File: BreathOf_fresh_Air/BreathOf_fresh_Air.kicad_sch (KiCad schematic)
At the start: 1 part, among them J1 4P4C

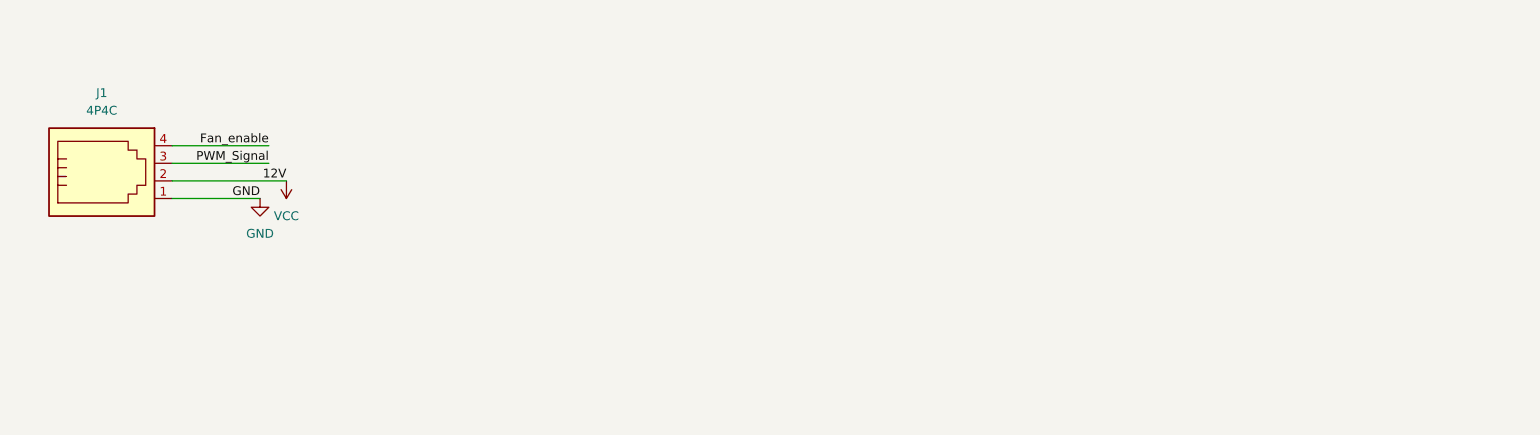
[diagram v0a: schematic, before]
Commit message: breath of fresh air
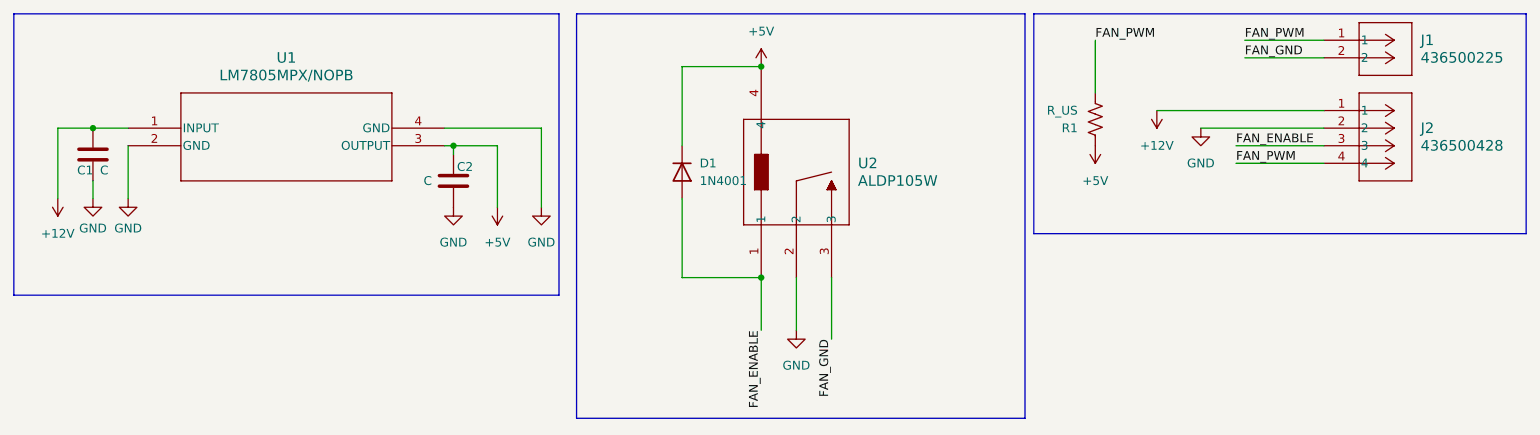
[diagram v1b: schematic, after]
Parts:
- removed J1: 4P4C, symbol Connector:4P4C
- added C1, C2: C, symbol Device:C
- added D1: 1N4001, Diode_THT:D_DO-41_SOD81_P10.16mm_Horizontal, symbol Diode:1N4001
- added J1: 436500225, CONN_SD-43650-009_02_MOL, symbol 43650-0225:436500225
- added J2: 436500428, CONN_SD-43650-010_04_MOL, symbol 43650-0428:436500428
- added R1: R_US, symbol Device:R_US
- added U1: LM7805MPX/NOPB, DCY4_TEX, symbol LM7805MPX/NOPB:LM7805MPX_NOPB
- added U2: ALDP105W, PAN_ALD_PAN, symbol ALDP105W:ALDP105W
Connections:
- net GND: now also C1.2, C2.2, J2.2, U1.2 (GND), U1.4 (GND), U2.2
- new net +12V: C1.1, J2.1, U1.1 (INPUT)
- new net +5V: C2.1, D1.1 (K), R1.1, U1.3 (OUTPUT), U2.4
- new net FAN_ENABLE: D1.2 (A), J2.3, U2.1
- new net FAN_GND: J1.2, U2.3
- new net FAN_PWM: J1.1, J2.4, R1.2
